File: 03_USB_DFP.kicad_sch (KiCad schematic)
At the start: 5 parts, among them U10 TPS20xxC, U11 TPS20xxC, U12 TPS20xxC, U8 TPS20xxC, U9 TPS20xxC

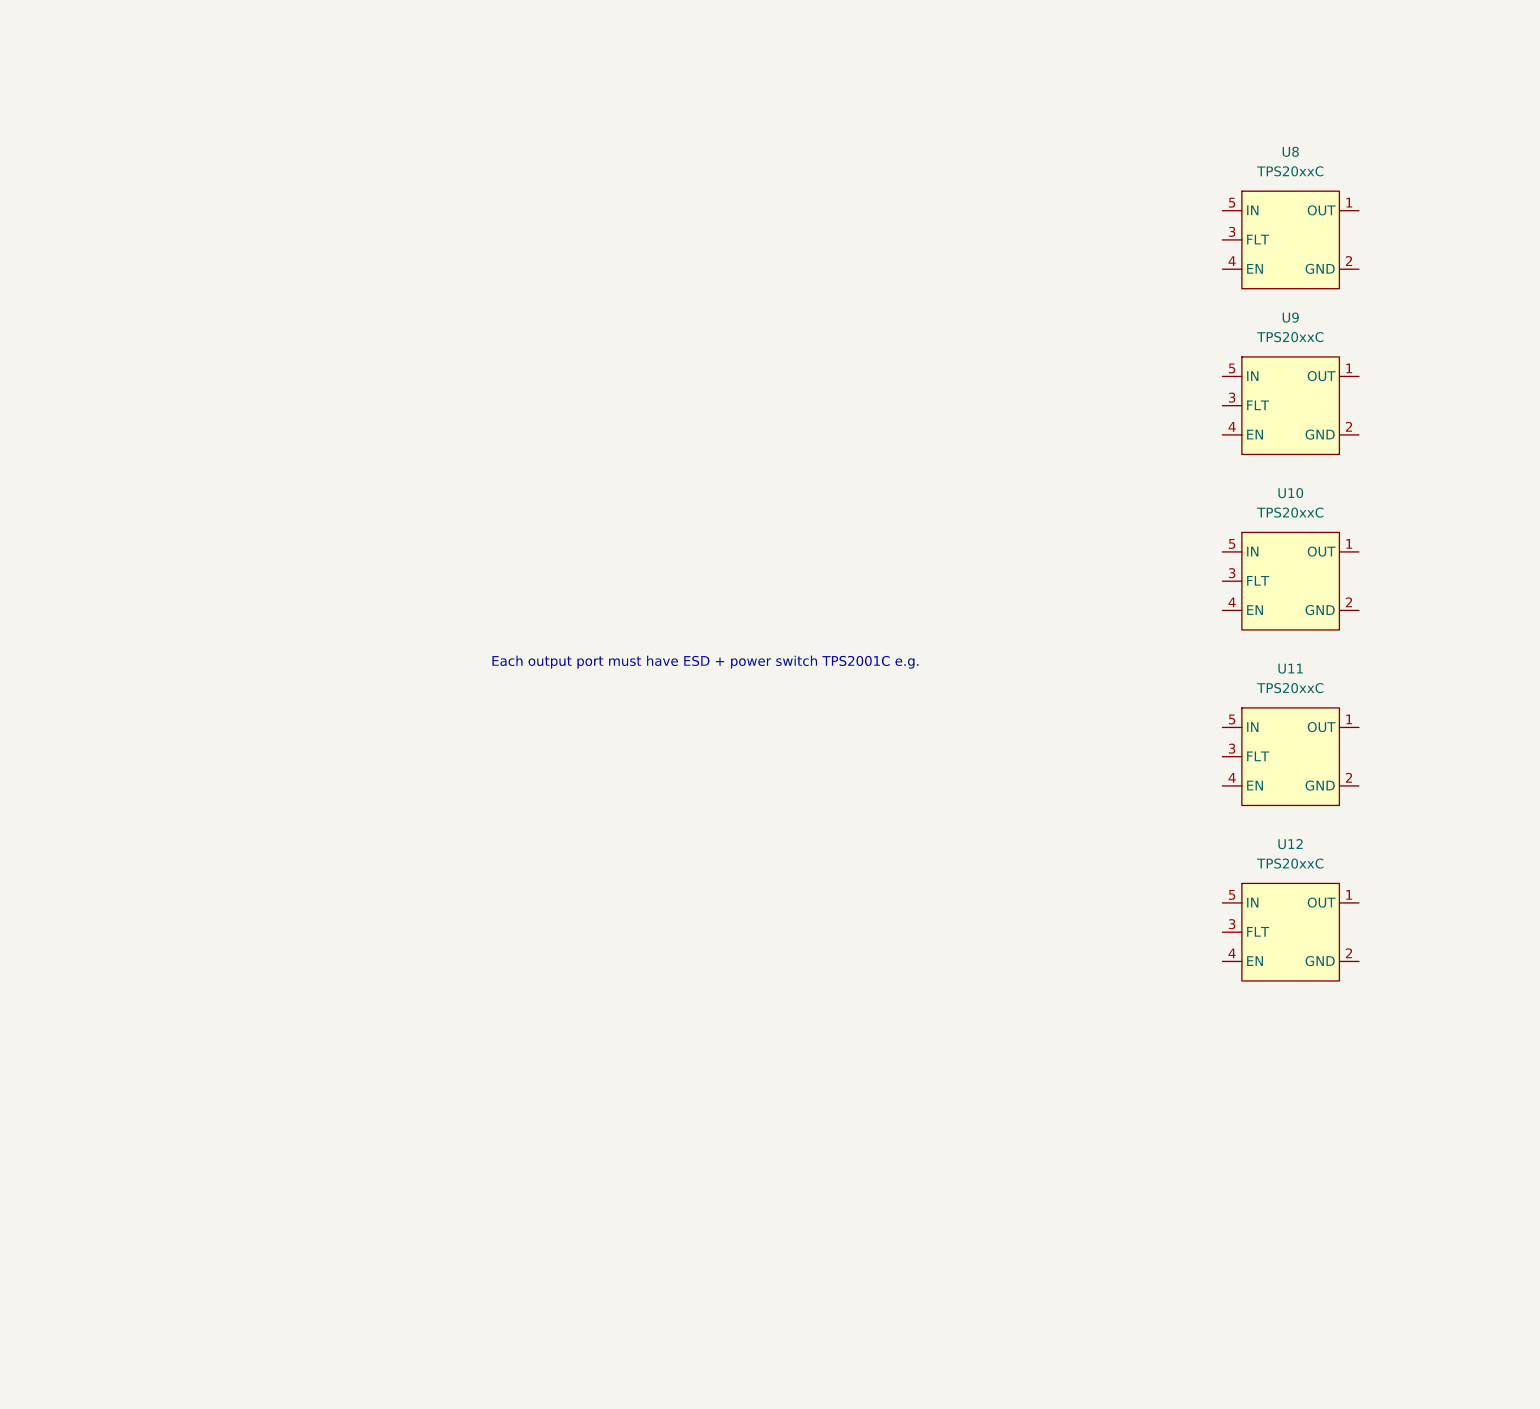
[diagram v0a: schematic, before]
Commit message: WIP hub and DFP
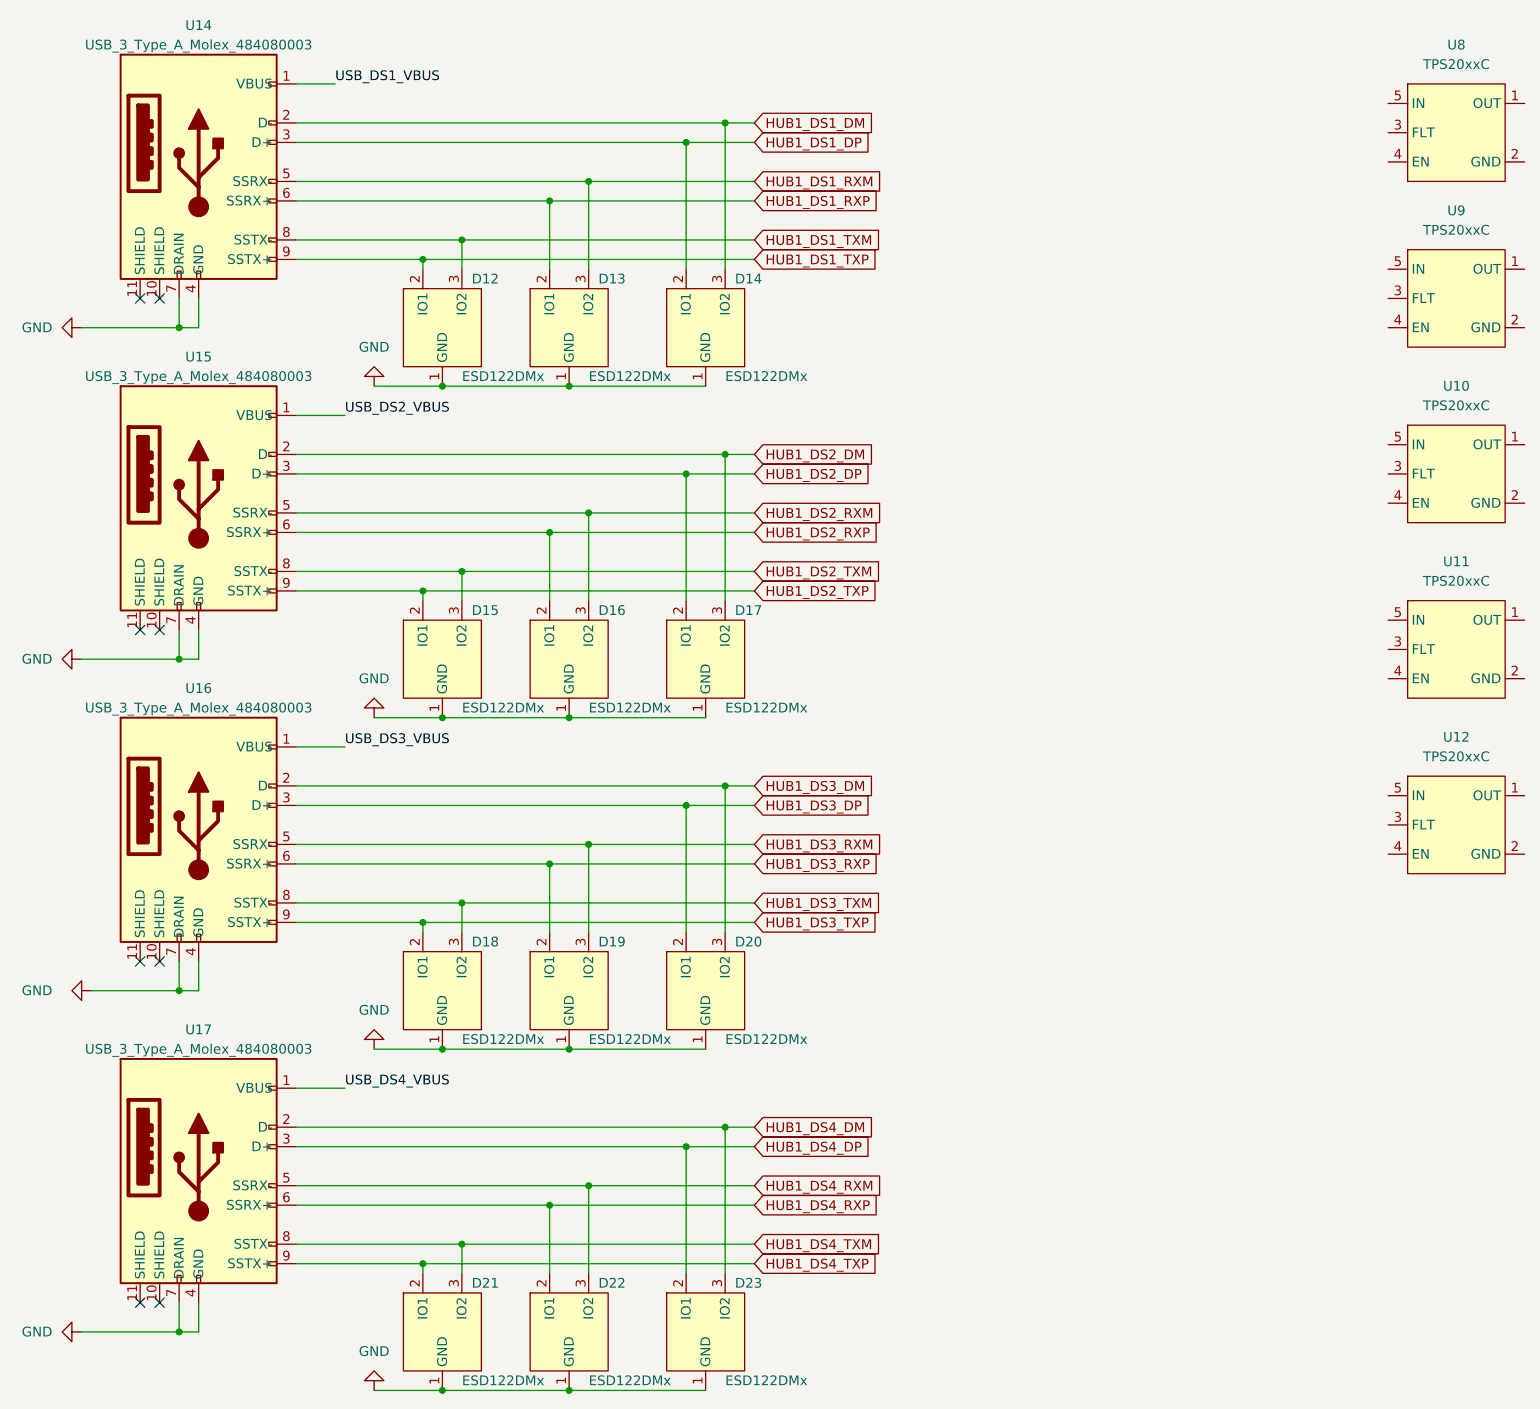
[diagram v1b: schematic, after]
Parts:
- added D12, D13, D14, D15, D16, D17, D18, D19, D20, D21, D22, D23: ESD122DMx, Cake_USB:ESD122DMX, symbol CakeUSB:ESD122DMx
- added U14, U15, U16, U17: USB_3_Type_A_Molex_484080003, Cake_USB:Molex_484080003, symbol CakeUSB:USB_3_Type_A_Molex_484080003
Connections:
- new net GND: D12.1 (GND), D13.1 (GND), D14.1 (GND), D15.1 (GND), D16.1 (GND), D17.1 (GND), D18.1 (GND), D19.1 (GND), D20.1 (GND), D21.1 (GND), D22.1 (GND), D23.1 (GND), U14.4 (GND), U14.7 (DRAIN), U15.4 (GND), U15.7 (DRAIN), U16.4 (GND), U16.7 (DRAIN), U17.4 (GND), U17.7 (DRAIN)
- new net HUB1_DS1_DM: D14.3 (IO2), U14.2 (D-)
- new net HUB1_DS1_DP: D14.2 (IO1), U14.3 (D+)
- new net HUB1_DS1_RXM: D13.3 (IO2), U14.5 (SSRX-)
- new net HUB1_DS1_RXP: D13.2 (IO1), U14.6 (SSRX+)
- new net HUB1_DS1_TXM: D12.3 (IO2), U14.8 (SSTX-)
- new net HUB1_DS1_TXP: D12.2 (IO1), U14.9 (SSTX+)
- new net HUB1_DS2_DM: D17.3 (IO2), U15.2 (D-)
- new net HUB1_DS2_DP: D17.2 (IO1), U15.3 (D+)
- new net HUB1_DS2_RXM: D16.3 (IO2), U15.5 (SSRX-)
- new net HUB1_DS2_RXP: D16.2 (IO1), U15.6 (SSRX+)
- new net HUB1_DS2_TXM: D15.3 (IO2), U15.8 (SSTX-)
- new net HUB1_DS2_TXP: D15.2 (IO1), U15.9 (SSTX+)
- new net HUB1_DS3_DM: D20.3 (IO2), U16.2 (D-)
- new net HUB1_DS3_DP: D20.2 (IO1), U16.3 (D+)
- new net HUB1_DS3_RXM: D19.3 (IO2), U16.5 (SSRX-)
- new net HUB1_DS3_RXP: D19.2 (IO1), U16.6 (SSRX+)
- new net HUB1_DS3_TXM: D18.3 (IO2), U16.8 (SSTX-)
- new net HUB1_DS3_TXP: D18.2 (IO1), U16.9 (SSTX+)
- new net HUB1_DS4_DM: D23.3 (IO2), U17.2 (D-)
- new net HUB1_DS4_DP: D23.2 (IO1), U17.3 (D+)
- new net HUB1_DS4_RXM: D22.3 (IO2), U17.5 (SSRX-)
- new net HUB1_DS4_RXP: D22.2 (IO1), U17.6 (SSRX+)
- new net HUB1_DS4_TXM: D21.3 (IO2), U17.8 (SSTX-)
- new net HUB1_DS4_TXP: D21.2 (IO1), U17.9 (SSTX+)
- new net USB_DS1_VBUS: U14.1 (VBUS)
- new net USB_DS2_VBUS: U15.1 (VBUS)
- new net USB_DS3_VBUS: U16.1 (VBUS)
- new net USB_DS4_VBUS: U17.1 (VBUS)
- no-connect marks 0 -> 8
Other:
- note removed: "Each output port must have ESD + power switch TPS2001C e.g."
- moved on the sheet: U10, U11, U12, U8, U9
